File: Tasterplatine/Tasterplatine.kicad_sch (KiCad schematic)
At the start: 3 parts, among them J1 2,5 MSFW 06, SW1 Marquardt 1010.8502

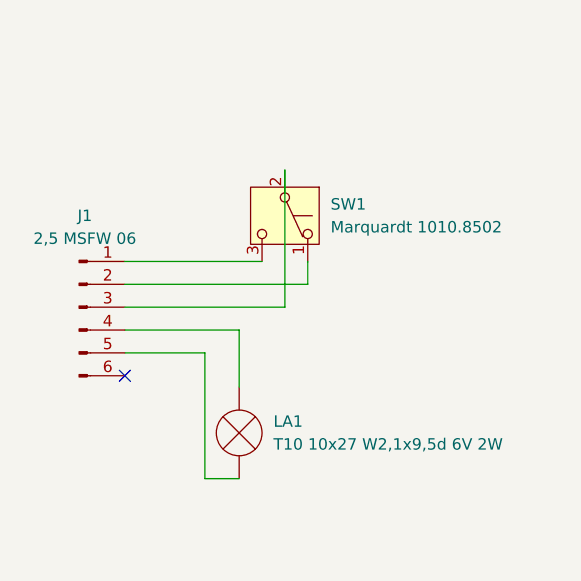
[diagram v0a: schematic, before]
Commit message: pins
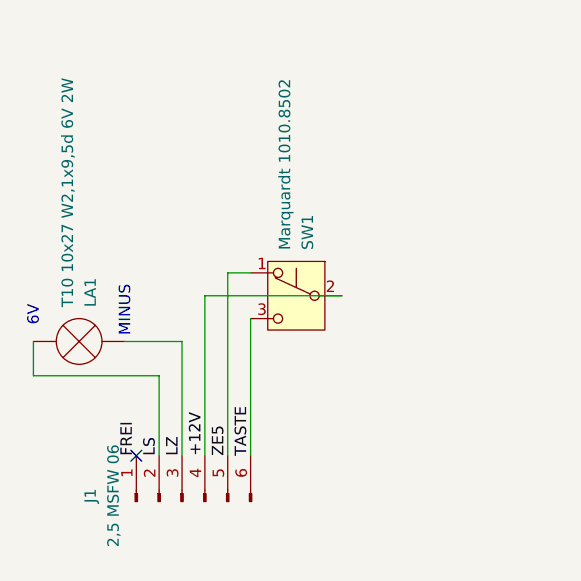
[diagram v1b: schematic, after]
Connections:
- net LS: now reaches LA1.1 (-)
- net LS: now also J1.2 (Pin_2); no longer J1.5 (Pin_5)
- net +12V: now reaches J1.4 (Pin_4)
- net +12V: now also SW1.2 (B); no longer LA1.2 (+)
- net ZE5: now reaches SW1.1 (A)
- net ZE5: now also J1.5 (Pin_5); no longer J1.2 (Pin_2)
- net LZ: now reaches J1.3 (Pin_3)
- net LZ: now also LA1.2 (+); no longer SW1.2 (B)
- net FREI: now reaches J1.1 (Pin_1)
- net FREI: no longer SW1.3 (C)
- net TASTE: now reaches J1.6 (Pin_6)
- net TASTE: now also SW1.3 (C)
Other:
- note added: "6V"
- note added: "MINUS"
- moved on the sheet: J1, LA1, SW1
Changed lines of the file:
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@@
 		(comment 1 "4079/030501/E")
 	)
+	(text "MINUS"
+		(exclude_from_sim no)
+		(at 74.93 57.658 90)
+		(effects
+			(font
+				(size 1.27 1.27)
+			)
+		)
+	)
+	(text "6V"
+		(exclude_from_sim no)
+		(at 64.77 58.166 90)
+		(effects
+			(font
+				(size 1.27 1.27)
+			)
+		)
+	)
 	(no_connect
-		(at 74.93 64.77)
-	)
-	(wire
-		(pts
-			(xy 87.63 59.69) (xy 87.63 66.04)
-		)
-		(stroke
-			(width 0)
-			(type default)
-		)
-	)
-	(wire
-		(pts
-			(xy 87.63 76.2) (xy 83.82 76.2)
-		)
-		(stroke
-			(width 0)
-			(type default)
-		)
-	)
-	(wire
-		(pts
-			(xy 92.71 57.15) (xy 92.71 41.91)
-		)
-		(stroke
-			(width 0)
-			(type default)
-		)
-	)
-	(wire
-		(pts
-			(xy 74.93 59.69) (xy 87.63 59.69)
-		)
-		(stroke
-			(width 0)
-			(type default)
-		)
-	)
-	(wire
-		(pts
-			(xy 83.82 62.23) (xy 74.93 62.23)
-		)
-		(stroke
-			(width 0)
-			(type default)
-		)
-	)
-	(wire
-		(pts
-			(xy 95.25 52.07) (xy 95.25 54.61)
-		)
-		(stroke
-			(width 0)
-			(type default)
-		)
-	)
-	(wire
-		(pts
-			(xy 95.25 54.61) (xy 74.93 54.61)
-		)
-		(stroke
-			(width 0)
-			(type default)
-		)
-	)
-	(wire
-		(pts
-			(xy 83.82 76.2) (xy 83.82 62.23)
-		)
-		(stroke
-			(width 0)
-			(type default)
-		)
-	)
-	(wire
-		(pts
-			(xy 74.93 57.15) (xy 92.71 57.15)
-		)
-		(stroke
-			(width 0)
-			(type default)
-		)
-	)
-	(wire
-		(pts
-			(xy 74.93 52.07) (xy 90.17 52.07)
-		)
-		(stroke
-			(width 0)
-			(type default)
+		(at 76.2 73.66)
+	)
+	(wire
+		(pts
+			(xy 81.28 60.96) (xy 74.93 60.96)
+		)
+		(stroke
+			(width 0)
+			(type default)
+		)
+	)
+	(wire
+		(pts
+			(xy 64.77 60.96) (xy 64.77 64.77)
+		)
+		(stroke
+			(width 0)
+			(type default)
+		)
+	)
+	(wire
+		(pts
+			(xy 83.82 55.88) (xy 99.06 55.88)
+		)
+		(stroke
+			(width 0)
+			(type default)
+		)
+	)
+	(wire
+		(pts
+			(xy 81.28 73.66) (xy 81.28 60.96)
+		)
+		(stroke
+			(width 0)
+			(type default)
+		)
+	)
+	(wire
+		(pts
+			(xy 78.74 64.77) (xy 78.74 73.66)
+		)
+		(stroke
+			(width 0)
+			(type default)
+		)
+	)
+	(wire
+		(pts
+			(xy 88.9 53.34) (xy 86.36 53.34)
+		)
+		(stroke
+			(width 0)
+			(type default)
+		)
+	)
+	(wire
+		(pts
+			(xy 86.36 53.34) (xy 86.36 73.66)
+		)
+		(stroke
+			(width 0)
+			(type default)
+		)
+	)
+	(wire
+		(pts
+			(xy 64.77 64.77) (xy 78.74 64.77)
+		)
+		(stroke
+			(width 0)
+			(type default)
+		)
+	)
+	(wire
+		(pts
+			(xy 83.82 73.66) (xy 83.82 55.88)
+		)
+		(stroke
+			(width 0)
+			(type default)
+		)
+	)
+	(wire
+		(pts
+			(xy 88.9 73.66) (xy 88.9 58.42)
+		)
+		(stroke
+			(width 0)
+			(type default)
+		)
+	)
+	(label "FREI"
+		(at 76.2 73.66 90)
+		(effects
+			(font
+				(size 1.27 1.27)
+			)
+			(justify left bottom)
+		)
+	)
+	(label "+12V"
+		(at 83.82 73.66 90)
+		(effects
+			(font
+				(size 1.27 1.27)
+			)
+			(justify left bottom)
+		)
+	)
+	(label "LS"
+		(at 78.74 73.66 90)
+		(effects
+			(font
+				(size 1.27 1.27)
+			)
+			(justify left bottom)
+		)
+	)
+	(label "TASTE"
+		(at 88.9 73.66 90)
+		(effects
+			(font
+				(size 1.27 1.27)
+			)
+			(justify left bottom)
+		)
+	)
+	(label "LZ"
+		(at 81.28 73.66 90)
+		(effects
+			(font
+				(size 1.27 1.27)
+			)
+			(justify left bottom)
+		)
+	)
+	(label "ZE5"
+		(at 86.36 73.66 90)
+		(effects
+			(font
+				(size 1.27 1.27)
+			)
+			(justify left bottom)
 		)
 	)
 	(symbol
 		(lib_id "Device:Lamp")
-		(at 87.63 71.12 0)
+		(at 69.85 60.96 270)
+		(mirror x)
 		(unit 1)
 		(exclude_from_sim no)
@@
 		(fields_autoplaced yes)
 		(property "Reference" "LA1"
-			(at 91.44 69.8499 0)
+			(at 71.1201 57.15 0)
 			(effects
 				(font
@@
 		)
 		(property "Value" "T10 10x27 W2,1x9,5d 6V 2W"
-			(at 91.44 72.3899 0)
+			(at 68.5801 57.15 0)
 			(effects
 				(font
@@
 		)
 		(property "Footprint" "Taster:LampSocket"
-			(at 87.63 68.58 90)
+			(at 72.39 60.96 90)
 			(effects
 				(font
@@
 		)
 		(property "Datasheet" "~"
-			(at 87.63 68.58 90)
+			(at 72.39 60.96 90)
 			(effects
 				(font
@@
 		)
 		(property "Description" "Lamp"
-			(at 87.63 71.12 0)
+			(at 69.85 60.96 0)
 			(effects
 				(font
@@
 	(symbol
 		(lib_id "Switch:SW_Push_SPDT")
-		(at 92.71 46.99 270)
+		(at 93.98 55.88 0)
+		(mirror y)
 		(unit 1)
 		(exclude_from_sim no)
@@
 		(fields_autoplaced yes)
 		(property "Reference" "SW1"
-			(at 97.79 45.7199 90)
+			(at 95.2501 50.8 90)
 			(effects
 				(font
@@
 		)
 		(property "Value" "Marquardt 1010.8502"
-			(at 97.79 48.2599 90)
+			(at 92.7101 50.8 90)
 			(effects
 				(font
@@
 		)
 		(property "Footprint" "Taster:Marquardt1010"
-			(at 92.71 46.99 0)
+			(at 93.98 55.88 0)
 			(effects
 				(font
@@
 		)
 		(property "Datasheet" "~"
-			(at 92.71 46.99 0)
+			(at 93.98 55.88 0)
 			(effects
 				(font
@@
 		)
 		(property "Description" "Momentary Switch, single pole double throw"
-			(at 92.71 46.99 0)
+			(at 93.98 55.88 0)
 			(effects
 				(font
@@
 	(symbol
 		(lib_id "Connector:Conn_01x06_Pin")
-		(at 69.85 57.15 0)
+		(at 81.28 78.74 90)
 		(unit 1)
 		(exclude_from_sim no)
@@
 		(on_board yes)
 		(dnp no)
-		(fields_autoplaced yes)
 		(property "Reference" "J1"
-			(at 70.485 46.99 0)
+			(at 71.12 78.105 0)
 			(effects
 				(font
@@
 		)
 		(property "Value" "2,5 MSFW 06"
-			(at 70.485 49.53 0)
+			(at 73.66 78.105 0)
 			(effects
 				(font
@@
 		)
 		(property "Footprint" "Connector_JST:JST_EH_S6B-EH_1x06_P2.50mm_Horizontal"
-			(at 69.85 57.15 0)
+			(at 81.28 78.74 0)
 			(effects
 				(font
@@
 		)
 		(property "Datasheet" "~"
-			(at 69.85 57.15 0)
+			(at 81.28 78.74 0)
 			(effects
 				(font
@@
 		)
 		(property "Description" "Generic connector, single row, 01x06, script generated"
-			(at 69.85 57.15 0)
-			(effects
-				(font
+			(at 81.28 78.74 0)
+			(effects
+				(font
